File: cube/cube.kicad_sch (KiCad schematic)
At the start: 112 parts, among them J1 Conn_01x08, J10 Conn_01x08, J2 Conn_01x08, J3 Conn_01x08, J4 Conn_01x08, J5 Conn_01x08, J6 Conn_01x08, J7 Conn_01x08, J8 Conn_01x08, J9 Conn_01x08, Q1 PN2222A, Q2 PN2222A, Q3 PN2222A, Q4 PN2222A, Q5 PN2222A, Q6 PN2222A, Q7 PN2222A, Q8 PN2222A, U1 74HC595, U2 74HC595, U3 74HC595, U4 74HC595, U5 74HC595, U6 74HC595, U7 74HC595, U8 74HC595, U9 74HC595

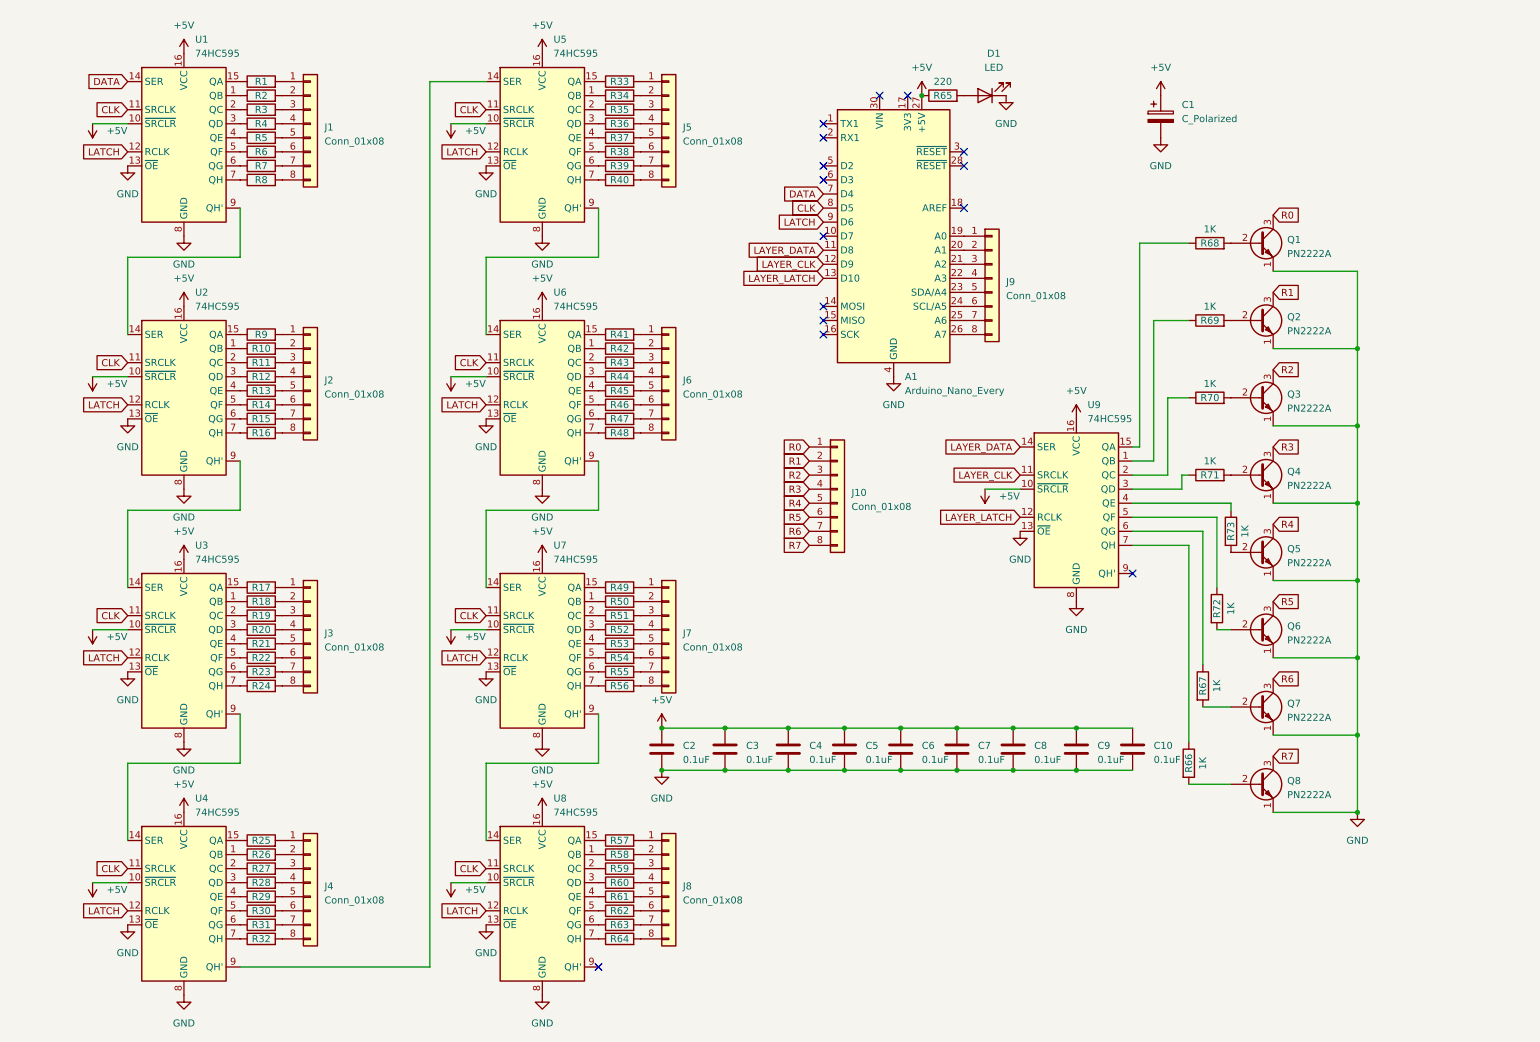
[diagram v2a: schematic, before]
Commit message: updated gerber files.
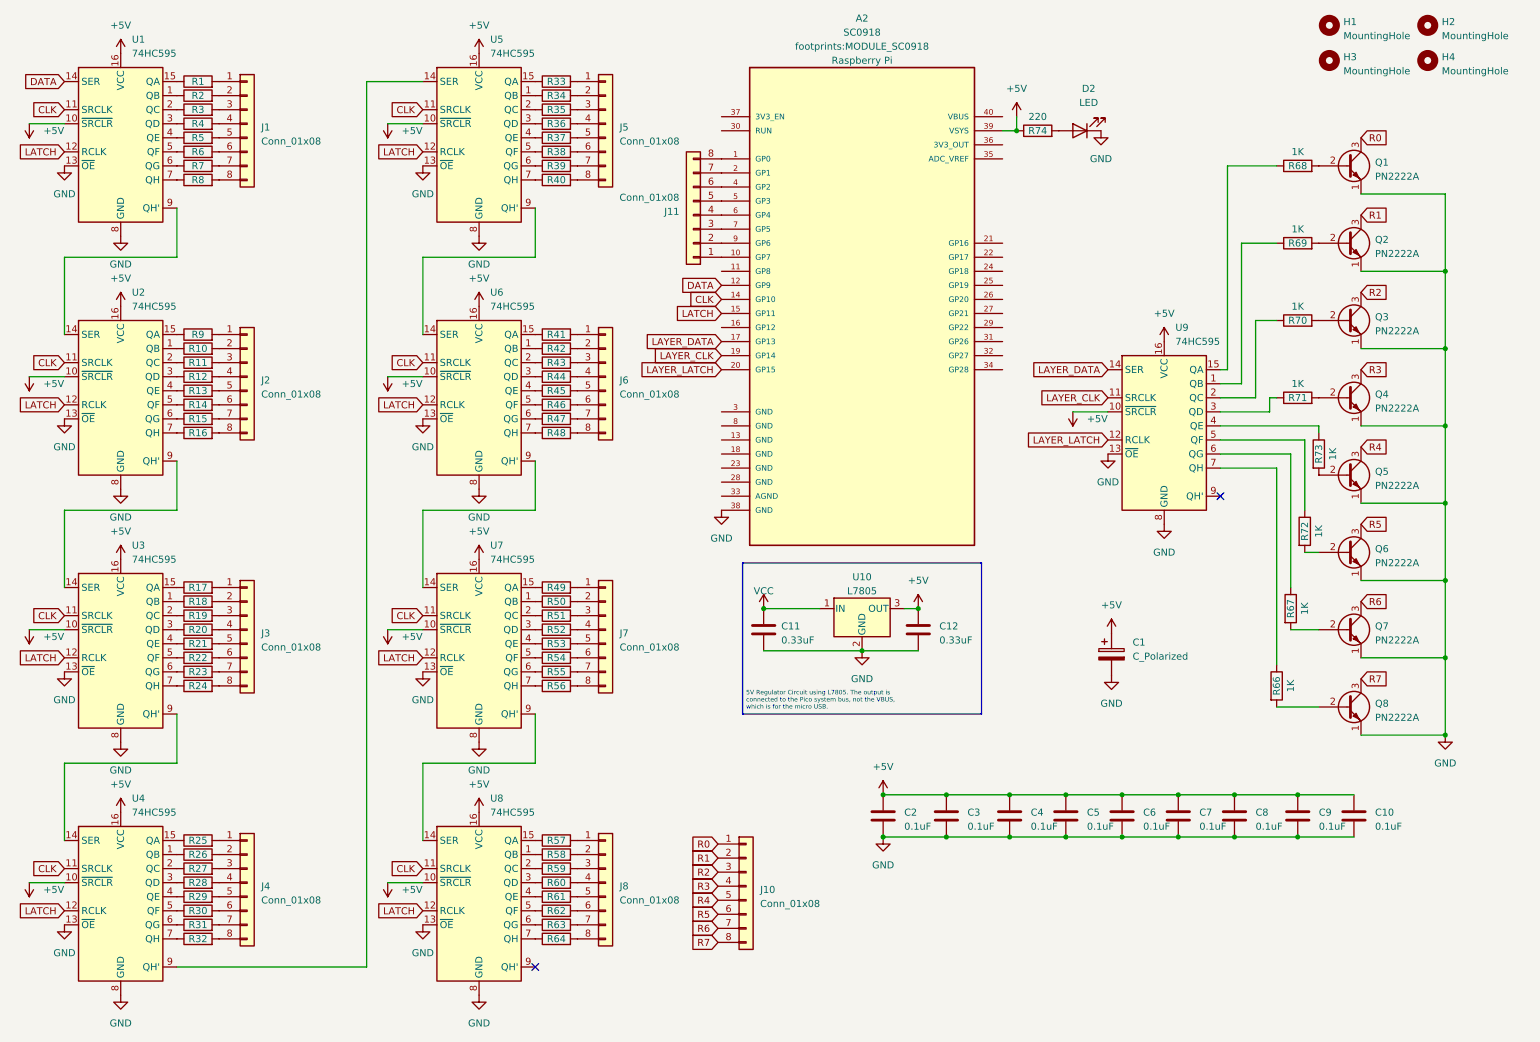
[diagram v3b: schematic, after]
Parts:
- removed A1: Arduino_Nano_Every, Module:Arduino_Nano, symbol MCU_Module:Arduino_Nano_Every
- removed D1: LED, LED_THT:LED_D5.0mm_Clear, symbol Device:LED
- removed J9: Conn_01x08, Connector_PinHeader_2.54mm:PinHeader_1x08_P2.54mm_Vertical, symbol Connector_Generic:Conn_01x08
- removed R65: 220, Resistor_THT:R_Axial_DIN0207_L6.3mm_D2.5mm_P10.16mm_Horizontal, symbol Device:R
- added A2: SC0918, footprints:MODULE_SC0918, symbol Raspberry_Pi_Pico_W_SC0918:SC0918
- added C11, C12: 0.33uF, Capacitor_THT:C_Disc_D5.1mm_W3.2mm_P5.00mm, symbol Device:C
- added D2: LED, LED_THT:LED_D5.0mm_Clear, symbol Device:LED
- added H1, H2, H3, H4: MountingHole, MountingHole:MountingHole_3.2mm_M3_DIN965_Pad, symbol Mechanical:MountingHole
- added J11: Conn_01x08, Connector_PinHeader_2.54mm:PinHeader_1x08_P2.54mm_Vertical, symbol Connector_Generic:Conn_01x08
- added R74: 220, Resistor_THT:R_Axial_DIN0207_L6.3mm_D2.5mm_P10.16mm_Horizontal, symbol Device:R
- added U10: L7805, Package_TO_SOT_THT:TO-220-3_Vertical, symbol Regulator_Linear:L7805
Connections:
- net +5V: now also A2.39 (VSYS), C12.1, R74.1, U10.3 (OUT)
- net CLK: now also A2.14 (GP10)
- net DATA: now also A2.12 (GP9)
- net GND: now also A2.38 (GND), C11.2, C12.2, D2.1 (K), U10.2 (GND)
- net LATCH: now also A2.15 (GP11)
- net LAYER_CLK: now also A2.19 (GP14)
- net LAYER_DATA: now also A2.17 (GP13)
- net LAYER_LATCH: now also A2.20 (GP15)
- new net: A2.10 (GP7), J11.1 (Pin_1)
- new net: A2.9 (GP6), J11.2 (Pin_2)
- new net: A2.7 (GP5), J11.3 (Pin_3)
- new net: A2.6 (GP4), J11.4 (Pin_4)
- new net: A2.5 (GP3), J11.5 (Pin_5)
- new net: A2.4 (GP2), J11.6 (Pin_6)
- new net: A2.2 (GP1), J11.7 (Pin_7)
- new net: A2.1 (GP0), J11.8 (Pin_8)
- new net: D2.2 (A), R74.2
- new net VCC: C11.1, U10.1 (IN)
- no-connect marks 15 -> 2
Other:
- note added: "5V Regulator Circuit using L7805. The output is connected to the Pico system bus, not the VBUS, which is for the micro USB."
- company: Marinkovic -> Strahinja Marinkovic
- moved on the sheet: C1, C10, C2, C3, C4, C5, C6, C7, C8, C9, J1, J10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
